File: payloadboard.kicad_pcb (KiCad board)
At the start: 2 copper layers, 46.8 x 46.8 mm, 12 parts, among them J1 TFM-110-12-L-D-A, J2 FLE-107-01-G-DV-A, U1 AP2112K-3.3

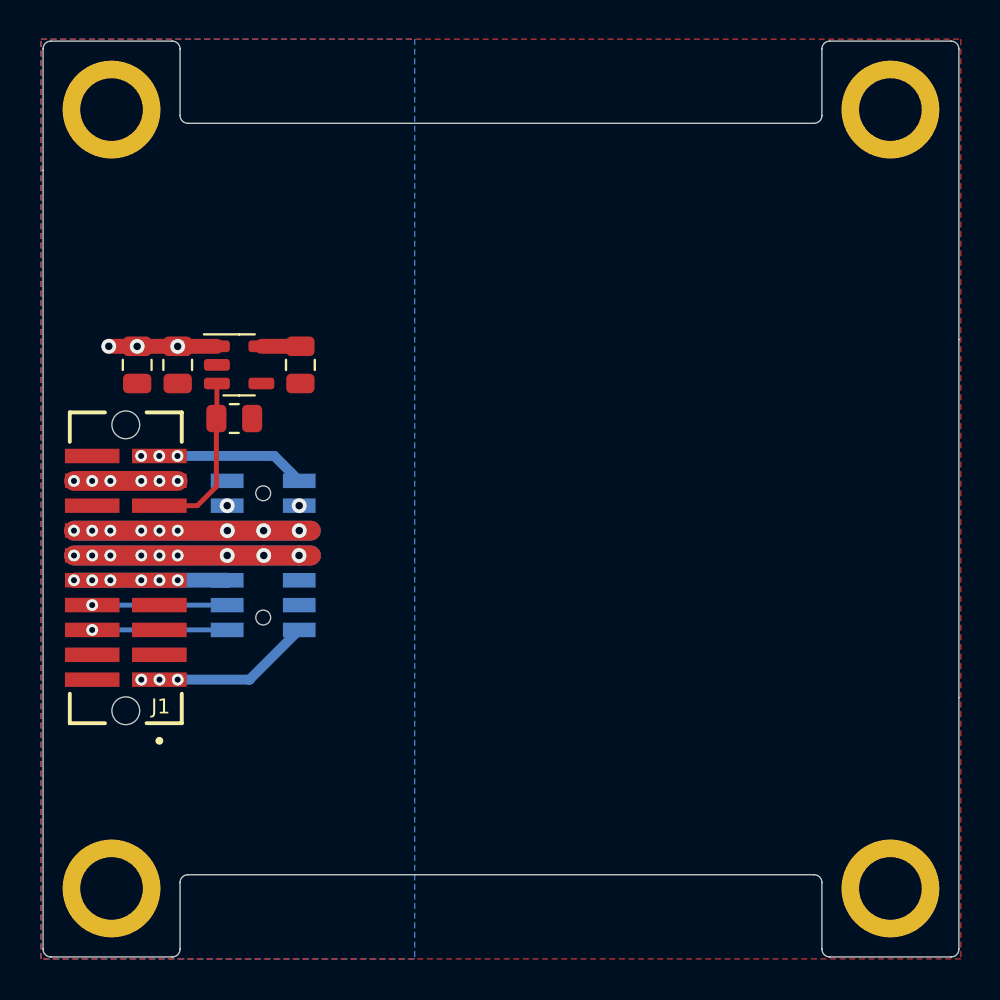
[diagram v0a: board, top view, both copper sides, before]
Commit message: Minor updates and export STEP / BOM
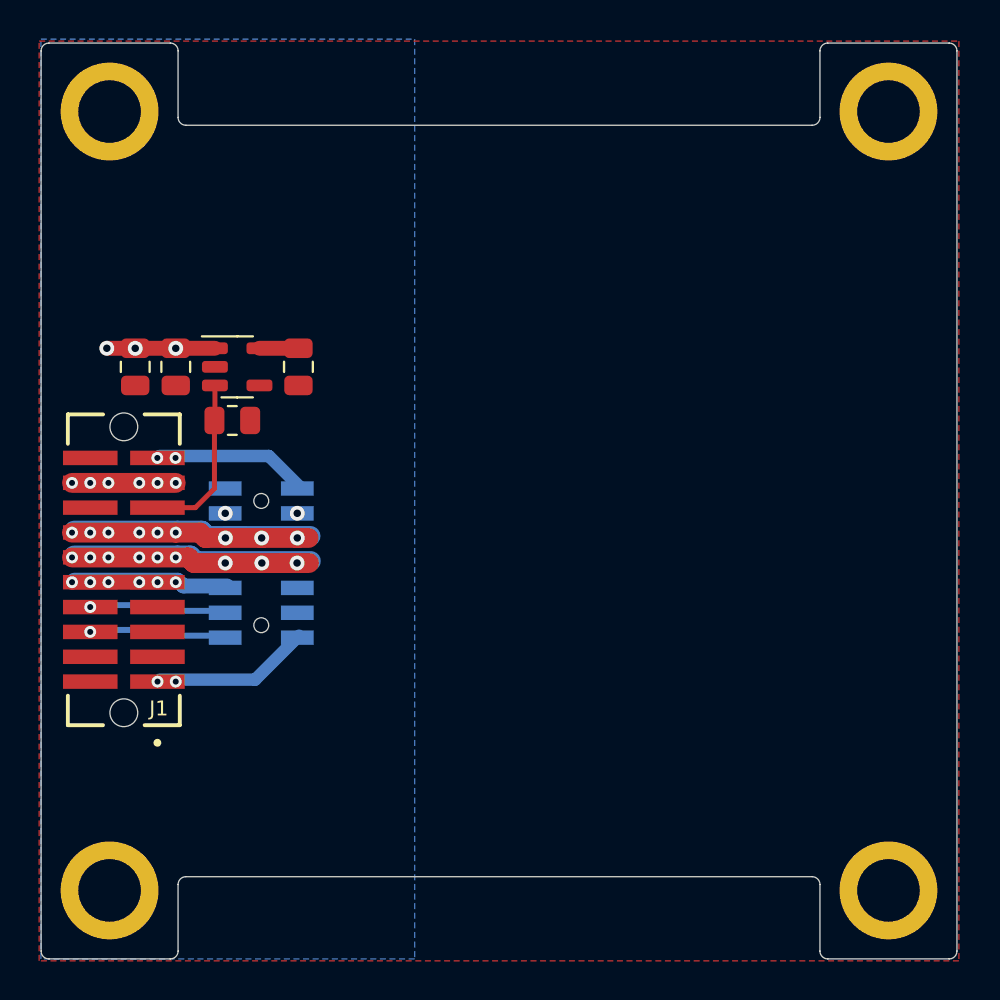
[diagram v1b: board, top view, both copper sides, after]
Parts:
- moved J2 0.40 mm to (95.1, 67.0)
- moved J1 0.14 mm to (88.1, 67.3)
- moved C2 0.14 mm to (90.8, 56.9)
- moved C3 0.14 mm to (97.0, 56.9)
- moved Ref** 0.14 mm to (107.8, 46.9)
- moved U1 0.14 mm to (93.9, 56.9)
- moved H1 0.14 mm to (87.4, 43.9)
- moved R1 0.14 mm to (93.7, 59.7)
- moved C1 0.14 mm to (88.7, 56.9)
- moved H4 0.14 mm to (87.4, 83.7)
- moved H2 0.14 mm to (127.2, 43.9)
- moved H3 0.14 mm to (127.2, 83.7)
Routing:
- net /COIL6_N: track 9.12 -> 8.07 mm, vias 3 -> 2
- net /BATT_P_SW: track 24.2 -> 25.2 mm
- net /BATT_N_SW: track 24.2 -> 25.2 mm
- net /COIL6_P: track 8.61 -> 7.80 mm, vias 3 -> 2
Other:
- outline, holes or cut-outs redrawn
- board text added: "06-NOV-22"
- board text removed: "09-OCT-22"
